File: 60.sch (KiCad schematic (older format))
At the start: 153 parts, among them K1 KEYSW, K10 KEYSW, K11 KEYSW, K12 KEYSW, K13 KEYSW, K14 KEYSW, K15 KEYSW, K16 KEYSW, K17 KEYSW, K18 KEYSW, K19 KEYSW, K2 KEYSW, K20 KEYSW, K21 KEYSW, K22 KEYSW, K23 KEYSW, K24 KEYSW, K25 KEYSW, K26 KEYSW, K27 KEYSW, K28 KEYSW, K29 KEYSW, K3 KEYSW, K30 KEYSW, K31 KEYSW, K32 KEYSW, K33 KEYSW, K34 KEYSW, K35 KEYSW, K36 KEYSW, K37 KEYSW, K38 KEYSW, K39 KEYSW, K4 KEYSW, K40 KEYSW, K41 KEYSW, K42 KEYSW, K43 KEYSW, K44 KEYSW, K45 KEYSW, K46 KEYSW, K47 KEYSW, K48 KEYSW, K49 KEYSW, K5 KEYSW, K50 KEYSW, K51 KEYSW, K52 KEYSW, K53 KEYSW, K54 KEYSW, K55 KEYSW, K56 KEYSW, K57 KEYSW, K58 KEYSW, K59 KEYSW, K6 KEYSW, K60 KEYSW, K61 KEYSW, K62 KEYSW, K63 KEYSW, K64 KEYSW, K65 KEYSW, K66 KEYSW, K67 KEYSW, K68 KEYSW, K69 KEYSW, K7 KEYSW, K70 KEYSW, K71 KEYSW, K72 KEYSW, K73 KEYSW, K74 KEYSW, K75 KEYSW, K76 KEYSW, K77 KEYSW, K78 KEYSW, K79 KEYSW, K8 KEYSW, K80 KEYSW, K81 KEYSW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

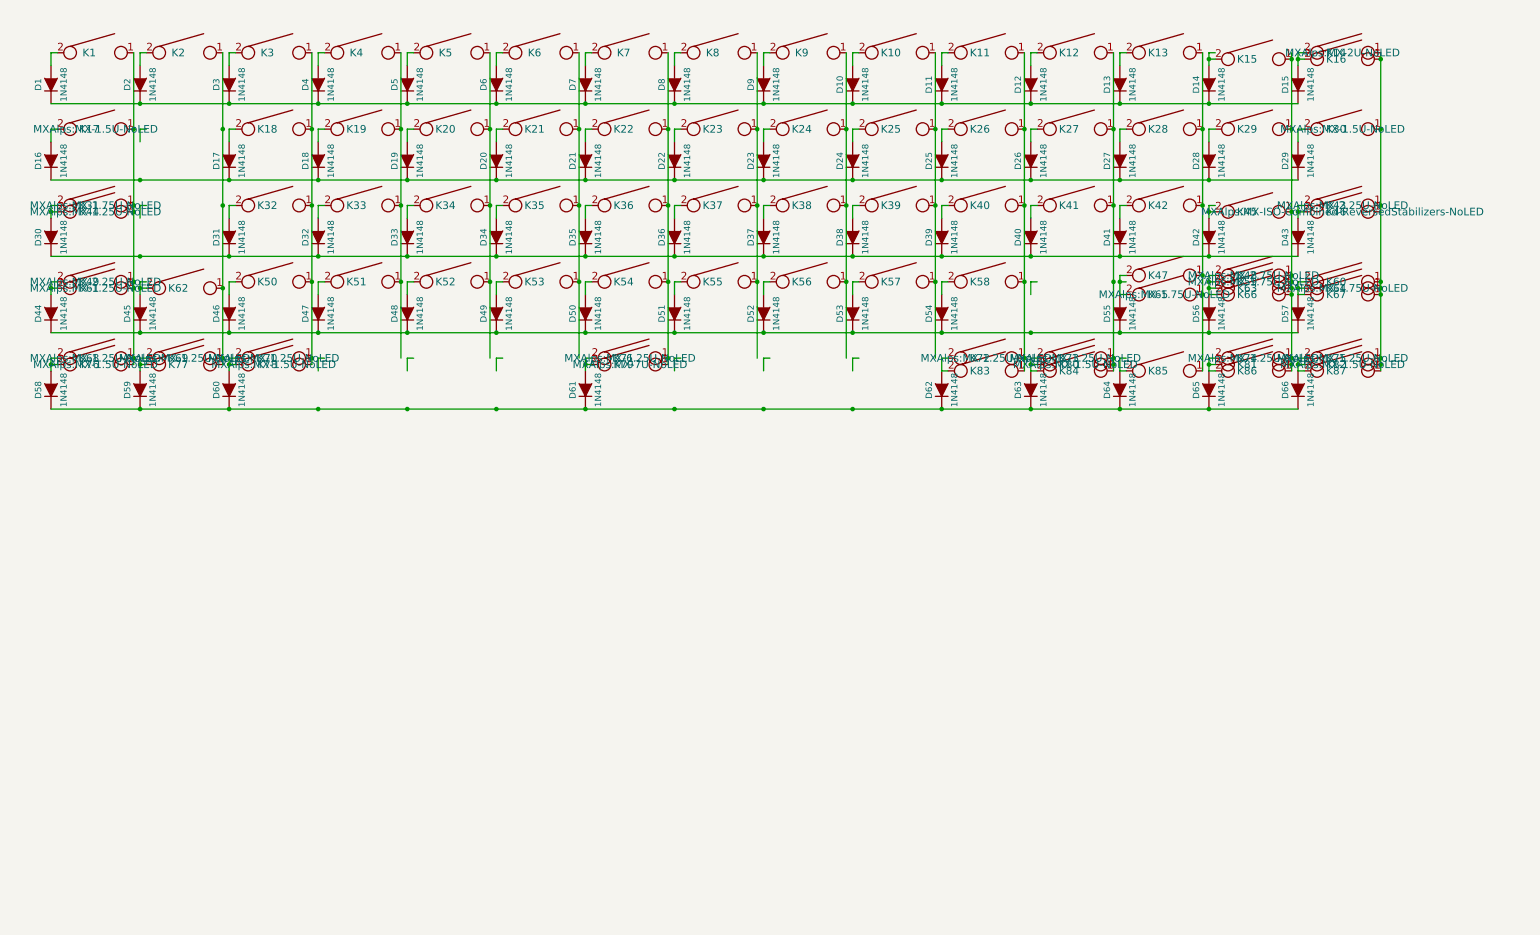
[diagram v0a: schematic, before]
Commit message: pre-diode swap
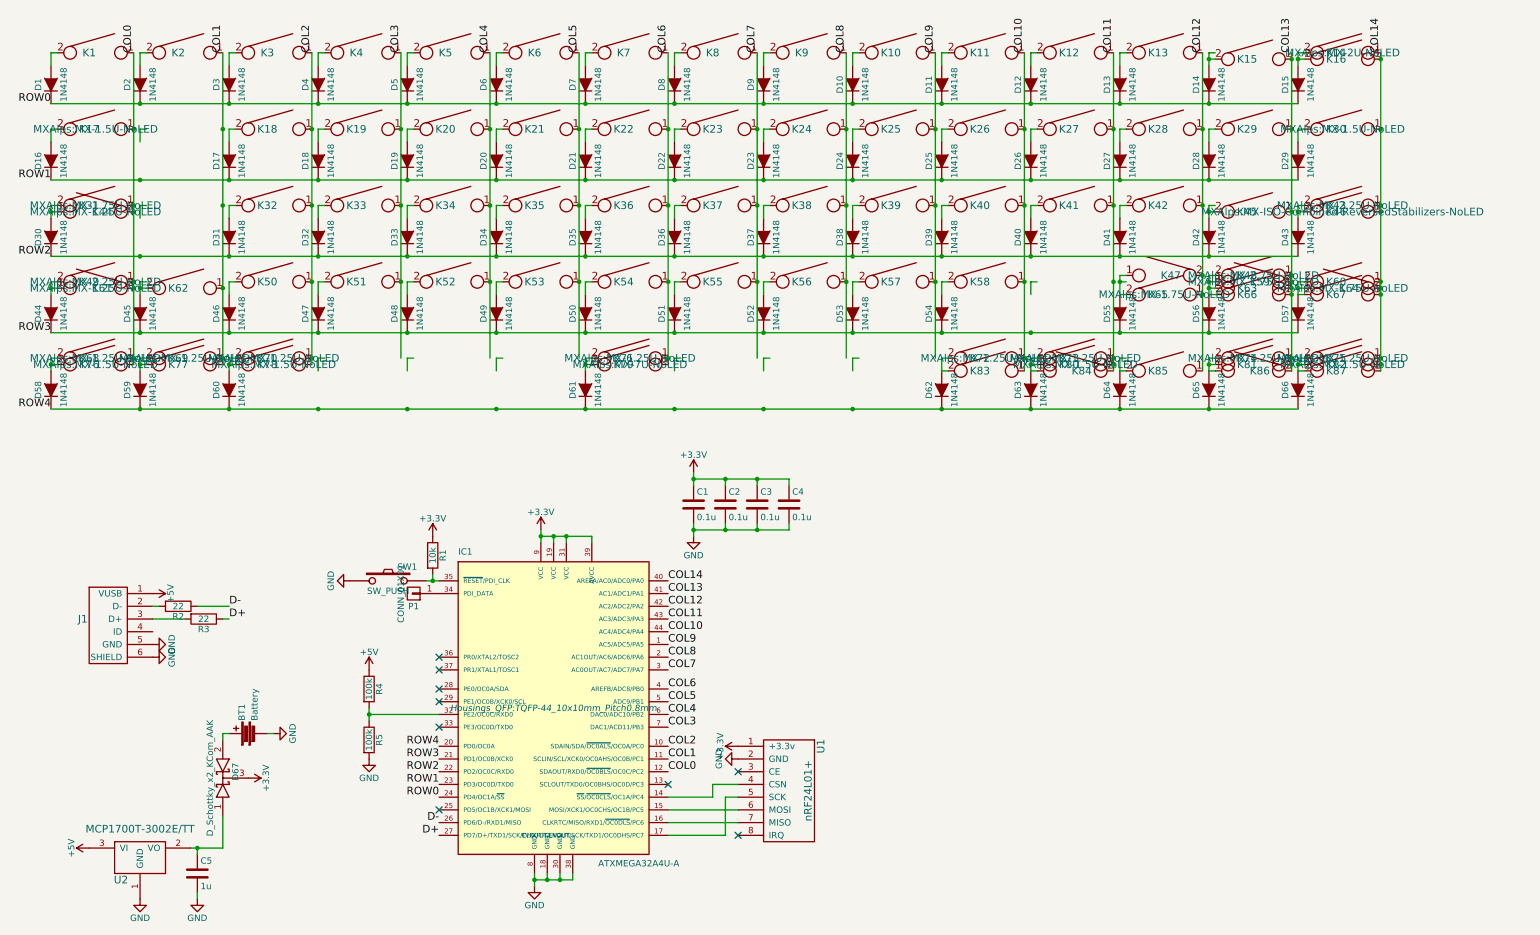
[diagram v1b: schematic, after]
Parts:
- added BT1: Battery, Battery_Holders:Keystone_1058_1x2032-CoinCell, symbol Battery
- added C1, C2, C3, C4: 0.1u, Capacitors_SMD:C_0805_HandSoldering, symbol C
- added C5: 1u, Capacitors_SMD:C_0805_HandSoldering, symbol C
- added D67: D_Schottky_x2_KCom_AAK, TO_SOT_Packages_SMD:SOT-23_Handsoldering, symbol D_Schottky_x2_KCom_AAK
- added IC1: ATXMEGA32A4U-A, Housings_QFP:TQFP-44_10x10mm_Pitch0.8mm, symbol ATXMEGA32A4U-A
- added J1: USB_mini_micro_B, symbol USB_mini_micro_B
- added P1: CONN_01X01, Connectors_TestPoints:Test_Point_Pad_d2.5mm, symbol CONN_01X01
- added R1: 10k, Resistors_SMD:R_0805_HandSoldering, symbol R
- added R2, R3: 22, Resistors_SMD:R_0805_HandSoldering, symbol R
- added R4, R5: 100k, Resistors_SMD:R_0805_HandSoldering, symbol R
- added SW1: SW_PUSH, Cartel:c&k_PTS645SH50SMTR92_LFS, symbol SW_PUSH
- added U1: nRF24L01+, Cartel:nRF24L01+_SMD, symbol nRF24L01+
- added U2: MCP1700T-3002E/TT, TO_SOT_Packages_SMD:SOT-23_Handsoldering, symbol MCP1700T-3002E/TT
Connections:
- net labels added: +3.3V, +5V, COL0, COL1, COL10, COL11, COL12, COL13, COL14, COL2, COL3, COL4, COL5, COL6, COL7, COL8, COL9, D+, D-, GND, ROW0, ROW1, ROW2, ROW3, ROW4
- wire segments 196 -> 239
- no-connect marks 0 -> 9
